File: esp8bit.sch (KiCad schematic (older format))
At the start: 10 parts, among them J1 Touchscreen, J2 Mini-DIN_6, J3 SD, J4 Sound, J5 Barrel_Jack_Switch, U1 WeMos_mini, U2 LM7805_TO220

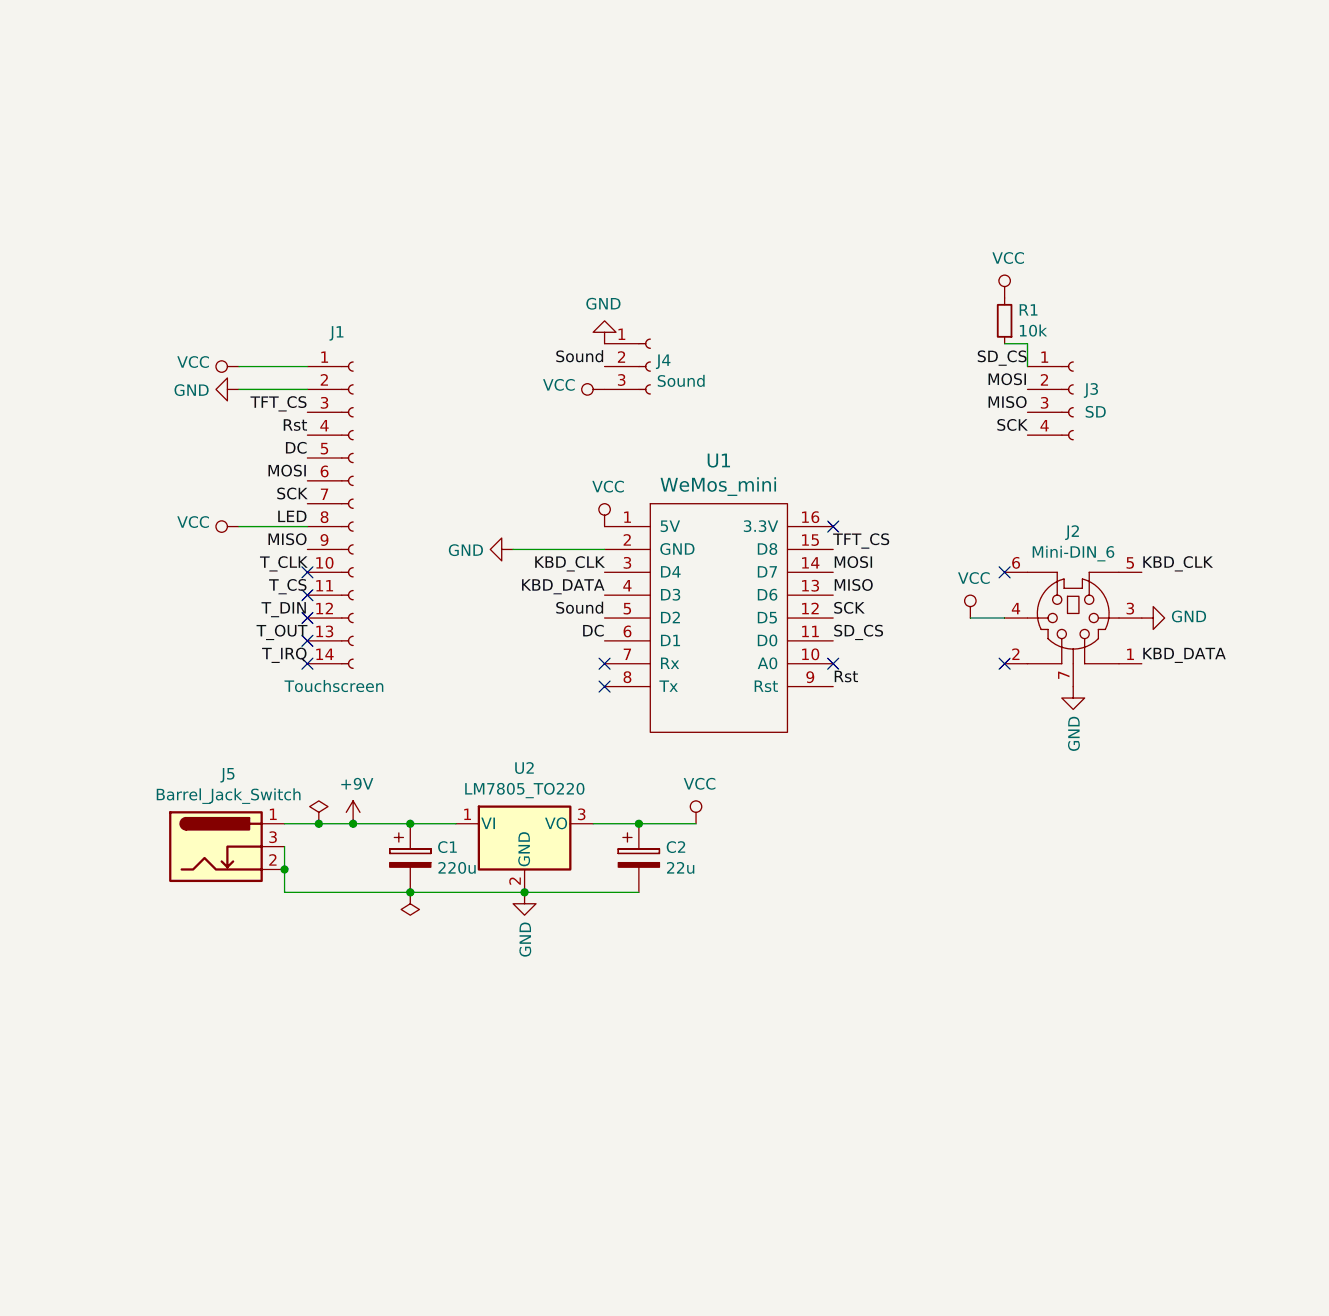
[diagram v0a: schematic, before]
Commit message: updates
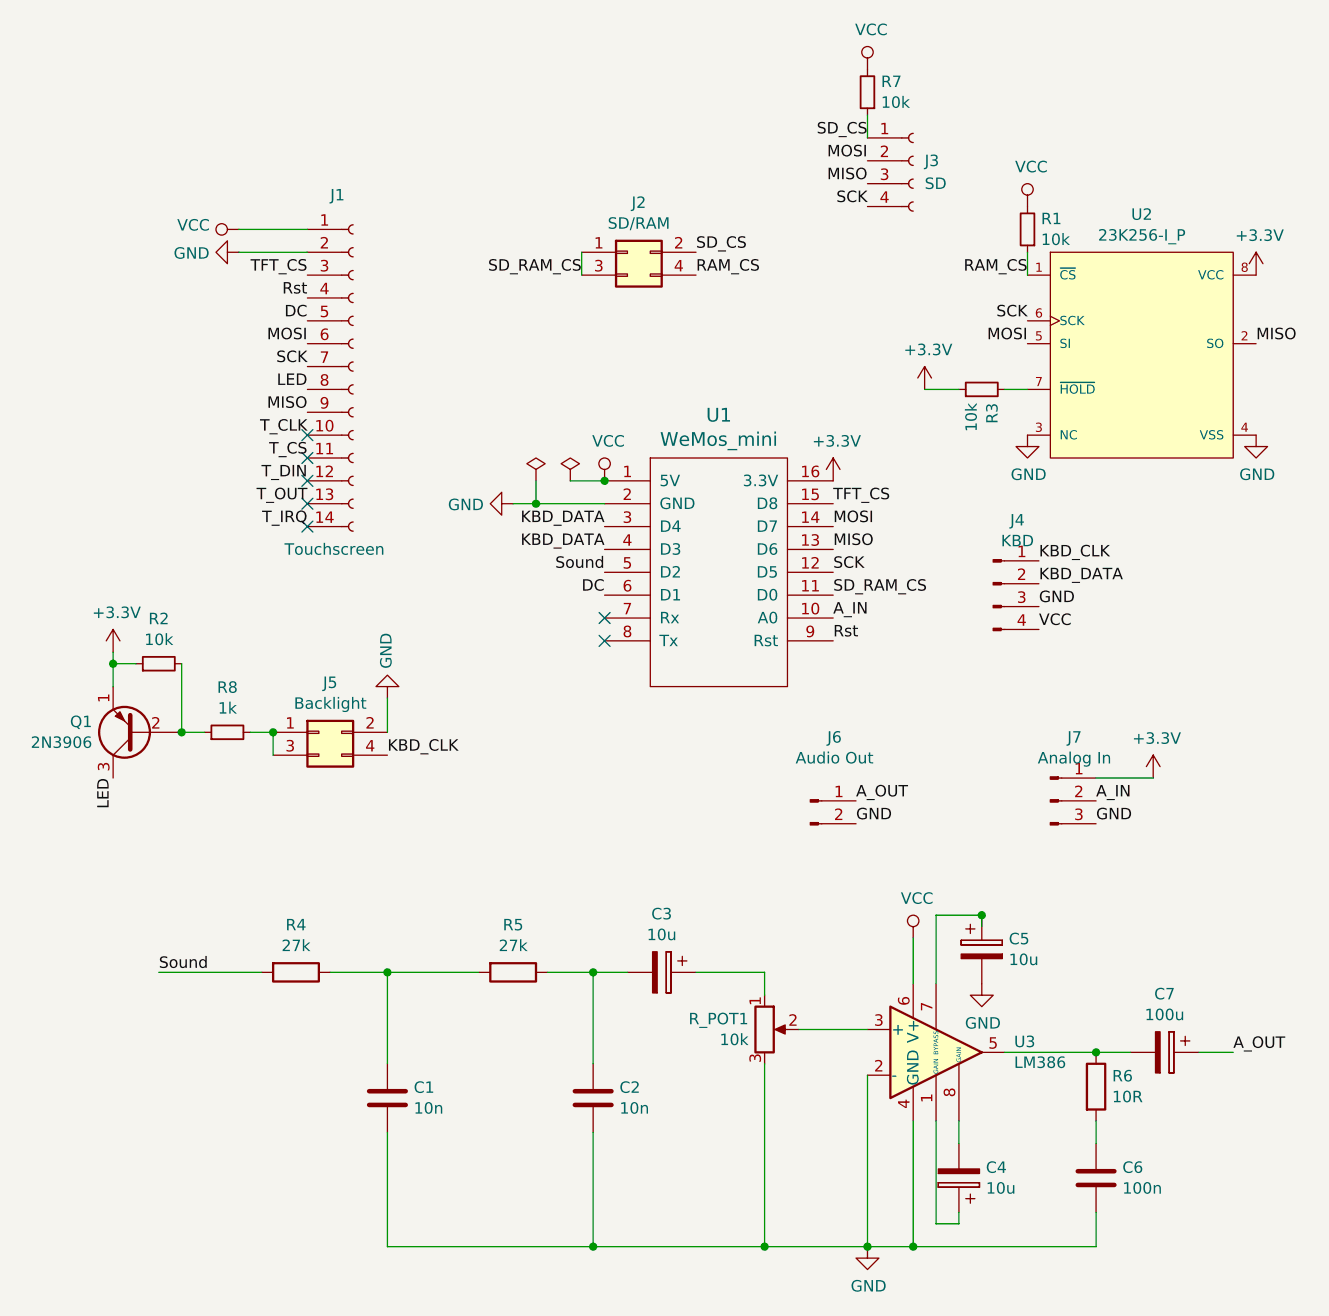
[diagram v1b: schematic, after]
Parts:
- removed C1: 220u, Capacitor_THT:CP_Radial_D6.3mm_P2.50mm, symbol Device:CP
- removed C2: 22u, Capacitor_THT:CP_Radial_D5.0mm_P2.50mm, symbol Device:CP
- removed J2: Mini-DIN_6, Custom_Footprints:Connector_Mini-DIN_Female_6Pin_2rows, symbol custom_symbols:Mini-DIN_6pins_ver3
- removed J4: Sound, Connector_PinHeader_2.54mm:PinHeader_1x03_P2.54mm_Vertical, symbol Connector:Conn_01x03_Female
- removed J5: Barrel_Jack_Switch, Connector_BarrelJack:BarrelJack_CUI_PJ-102AH_Horizontal, symbol Connector:Barrel_Jack_Switch
- removed U2: LM7805_TO220, Package_TO_SOT_THT:TO-220-3_Horizontal_TabDown, symbol Regulator_Linear:LM7805_TO220
- added C1, C2: 10n, Capacitor_THT:C_Disc_D6.0mm_W2.5mm_P5.00mm, symbol Device:C
- added C3, C4, C5: 10u, Capacitor_THT:CP_Radial_D5.0mm_P2.00mm, symbol Device:CP
- added C6: 100n, Capacitor_THT:C_Disc_D6.0mm_W2.5mm_P5.00mm, symbol Device:C
- added C7: 100u, Capacitor_THT:CP_Radial_D5.0mm_P2.00mm, symbol Device:CP
- added J2: SD/RAM, Connector_PinHeader_2.54mm:PinHeader_2x02_P2.54mm_Vertical, symbol Connector_Generic:Conn_02x02_Odd_Even
- added J4: KBD, Connector_PinHeader_2.54mm:PinHeader_1x04_P2.54mm_Horizontal, symbol Connector:Conn_01x04_Male
- added J5: Backlight, Connector_PinHeader_2.54mm:PinHeader_2x02_P2.54mm_Vertical, symbol Connector_Generic:Conn_02x02_Odd_Even
- added J6: Audio Out, Connector_PinHeader_2.54mm:PinHeader_1x02_P2.54mm_Horizontal, symbol Connector:Conn_01x02_Male
- added J7: Analog In, Connector_PinHeader_2.54mm:PinHeader_1x03_P2.54mm_Horizontal, symbol Connector:Conn_01x03_Male
- added Q1: 2N3906, Package_TO_SOT_THT:TO-92_HandSolder, symbol Device:Q_PNP_EBC
- added R2, R3, R7: 10k, Resistor_THT:R_Axial_DIN0207_L6.3mm_D2.5mm_P10.16mm_Horizontal, symbol Device:R_Small
- added R4, R5: 27k, Resistor_THT:R_Axial_DIN0207_L6.3mm_D2.5mm_P10.16mm_Horizontal, symbol Device:R
- added R6: 10R, Resistor_THT:R_Axial_DIN0207_L6.3mm_D2.5mm_P10.16mm_Horizontal, symbol Device:R
- added R8: 1k, Resistor_THT:R_Axial_DIN0207_L6.3mm_D2.5mm_P10.16mm_Horizontal, symbol Device:R_Small
- added R_POT1: 10k, Potentiometer_THT:Potentiometer_Bourns_3386P_Vertical, symbol Device:R_POT
- added U2: 23K256-I_P, Package_DIP:DIP-8_W7.62mm_Socket, symbol eec:23K256-I_P
- added U3: LM386, Package_DIP:DIP-8_W7.62mm_Socket, symbol Amplifier_Audio:LM386
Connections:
- net GND: now also C1.2, C2.2, C5.2, C6.2, J4.3 (Pin_3), J5.2 (Pin_2), J6.2 (Pin_2), J7.3 (Pin_3), R_POT1.3, U2.3 (NC), U2.4 (VSS), U3.2 (-), U3.4 (GND)
- net KBD_CLK: now also J4.1 (Pin_1), J5.4 (Pin_4); no longer U1.3 (D4)
- net KBD_DATA: now also U1.3 (D4), J4.2 (Pin_2)
- net MISO: now also U2.2 (SO)
- net MOSI: now also U2.5 (SI)
- net SCK: now also U2.6 (SCK)
- net SD_CS: now also J2.2 (Pin_2), R7.1; no longer R1.1, U1.11 (D0)
- net Sound: now also R4.2
- net VCC: now also J4.4 (Pin_4), R7.2, U3.6 (V+); no longer J1.8 (Pin_8)
- net A_IN: now reaches U1.10 (A0)
- net A_IN: now also J7.2 (Pin_2)
- net +3V3: now reaches U1.16 (3.3V)
- net +3V3: now also J7.1 (Pin_1), Q1.1 (E), R2.1, R3.1, U2.8 (VCC)
- new net: J5.1 (Pin_1), J5.3 (Pin_3), R8.2
- new net: R3.2, U2.7 (~HOLD~)
- new net: C4.1, U3.1 (GAIN)
- new net: R_POT1.2, U3.3 (+)
- new net: C7.2, R6.1, U3.5
- new net: C5.1, U3.7 (BYPASS)
- new net: C4.2, U3.8 (GAIN)
- new net: C6.1, R6.2
- new net: C3.1, R_POT1.1
- new net: C2.1, C3.2, R5.1
- new net: C1.1, R4.1, R5.2
- new net: Q1.2 (B), R2.2, R8.1
- new net A_OUT: C7.1, J6.1 (Pin_1)
- new net LED: J1.8 (Pin_8), Q1.3 (C)
- new net RAM_CS: J2.4 (Pin_4), R1.1, U2.1 (~CS~)
- new net SD_RAM_CS: J2.1 (Pin_1), J2.3 (Pin_3), U1.11 (D0)
- no-connect marks 11 -> 7
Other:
- moved on the sheet: J1, J3, R1, U1
